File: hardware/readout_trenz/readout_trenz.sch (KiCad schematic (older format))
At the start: 1 part, among them J1 Conn_02x05_Odd_Even

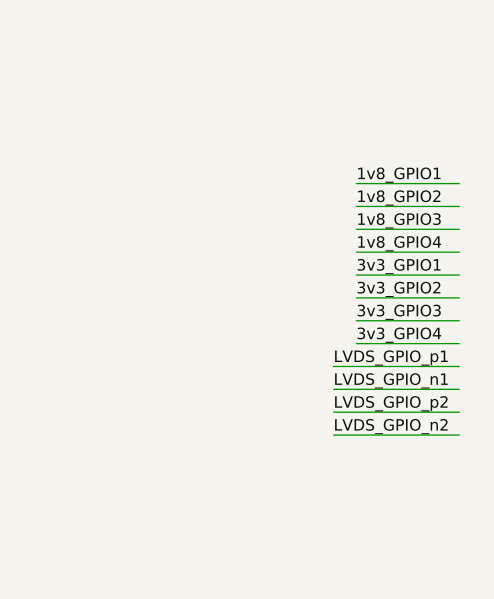
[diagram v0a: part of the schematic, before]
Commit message: Layout Started
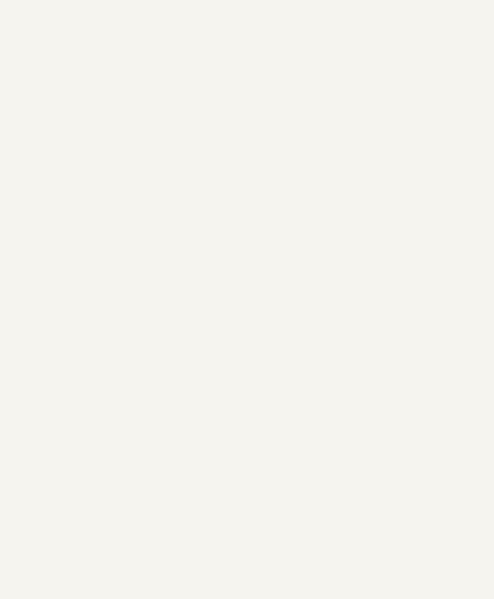
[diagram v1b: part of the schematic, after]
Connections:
- net labels removed: 1v8_GPIO1, 1v8_GPIO2, 1v8_GPIO3, 1v8_GPIO4, 3v3_GPIO1, 3v3_GPIO2, 3v3_GPIO3, 3v3_GPIO4, LVDS_GPIO_n1, LVDS_GPIO_n2, LVDS_GPIO_p1, LVDS_GPIO_p2
- wire segments 35 -> 23
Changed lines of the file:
@@
 Text Label 2550 4500 0    50   ~ 0
 B2_[0..31]
-Text Label 11550 5250 0    50   ~ 0
-LVDS_GPIO_n2
-Wire Wire Line
-	12100 5150 11550 5150
-Wire Wire Line
-	11550 5250 12100 5250
-Wire Wire Line
-	12100 4650 11650 4650
-Wire Wire Line
-	11650 4550 12100 4550
-Text Label 11650 4650 0    50   ~ 0
-3v3_GPIO2
-Text Label 11650 4550 0    50   ~ 0
-3v3_GPIO1
-Wire Wire Line
-	12100 4850 11650 4850
-Wire Wire Line
-	11650 4750 12100 4750
-Text Label 11650 4850 0    50   ~ 0
-3v3_GPIO4
-Text Label 11650 4750 0    50   ~ 0
-3v3_GPIO3
-Text Label 11550 5150 0    50   ~ 0
-LVDS_GPIO_p2
-Wire Wire Line
-	11550 5050 12100 5050
-Wire Wire Line
-	12100 4950 11550 4950
-Text Label 11550 5050 0    50   ~ 0
-LVDS_GPIO_n1
-Text Label 11550 4950 0    50   ~ 0
-LVDS_GPIO_p1
-Wire Wire Line
-	12100 4250 11650 4250
-Wire Wire Line
-	11650 4150 12100 4150
-Text Label 11650 4250 0    50   ~ 0
-1v8_GPIO2
-Text Label 11650 4150 0    50   ~ 0
-1v8_GPIO1
-Wire Wire Line
-	12100 4450 11650 4450
-Wire Wire Line
-	11650 4350 12100 4350
-Text Label 11650 4450 0    50   ~ 0
-1v8_GPIO4
-Text Label 11650 4350 0    50   ~ 0
-1v8_GPIO3
 Wire Wire Line
 	2500 6000 3500 6000
